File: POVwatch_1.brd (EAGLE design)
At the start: 25.4 x 36.8 mm, 48 parts, among them Q1 S8050, U1 ATMEGA168P-AU, U2 ADXL345, U3 MCP6001-SOT23, U4 APDS-9008, U5 TP4056, U6 3.3V, Y1 7.3728MHz

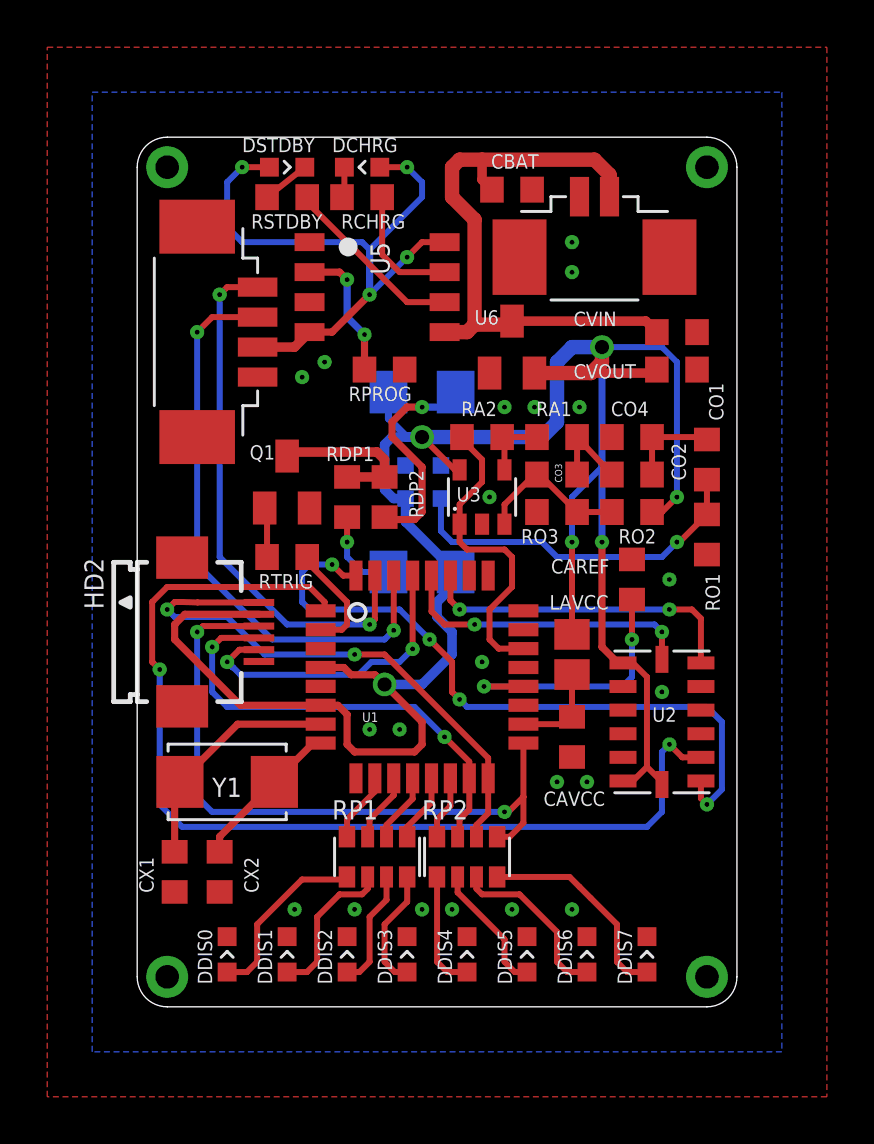
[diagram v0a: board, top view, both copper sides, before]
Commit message: This is POVwatch 1.0M
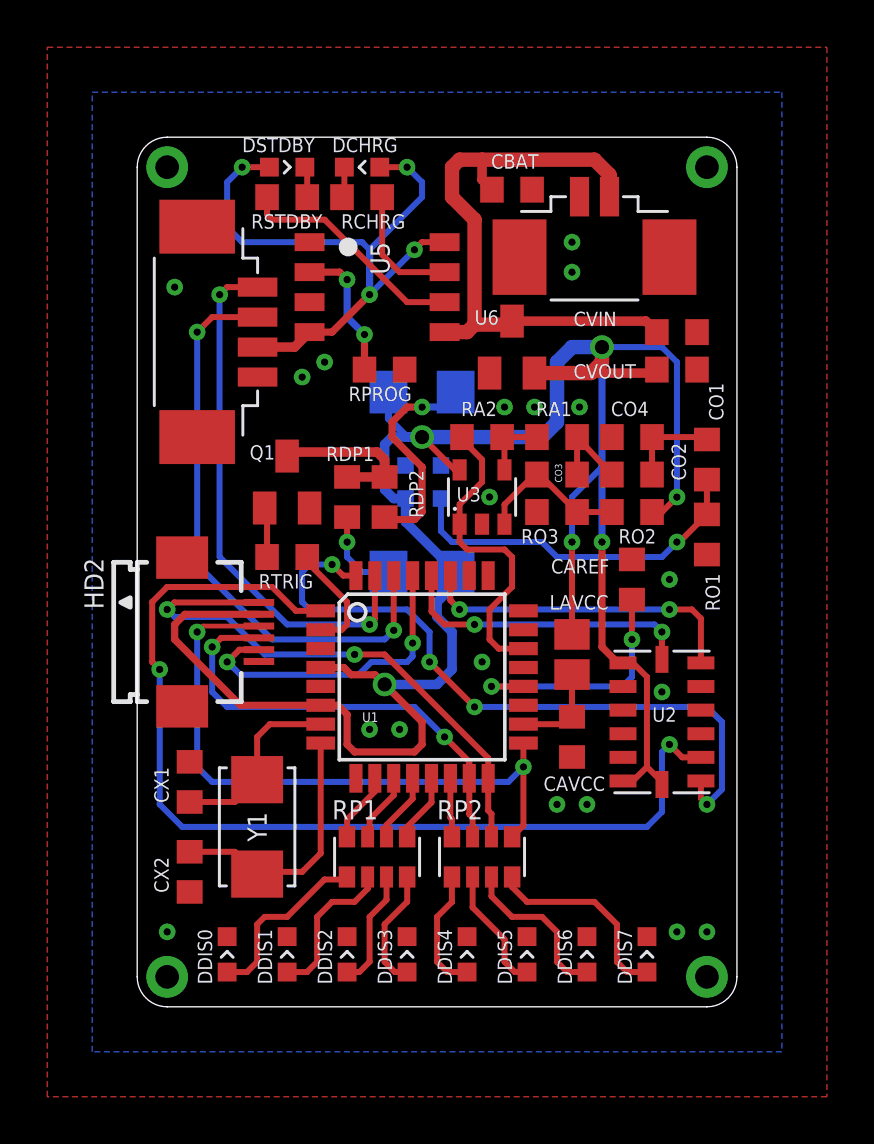
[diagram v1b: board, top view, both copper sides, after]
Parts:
- moved CX1 3.86 mm to (2.22, 9.53), turned to 270 degrees
- moved Y1 2.29 mm to (5.08, 7.62), turned to 270 degrees
- moved CX2 1.27 mm to (2.22, 5.71)
- moved RP2 0.63 mm to (14.6, 6.35)
- turned RSTDBY to 0 degrees
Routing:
- net X2: track 6.56 -> 11.0 mm
- net X1: track 10.0 -> 7.98 mm
- net STDBY: track 7.79 -> 9.79 mm
- net SCK/DIS7: track 28.8 -> 26.9 mm
- net STDBYR: track 2.04 -> 1.37 mm
- net AREF: track 11.4 -> 10.7 mm
